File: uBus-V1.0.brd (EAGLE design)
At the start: 160 x 100 mm, 20 parts, among them J1 FTDI, U1 MIC5219 3.3V, U2 FTS31XS-U

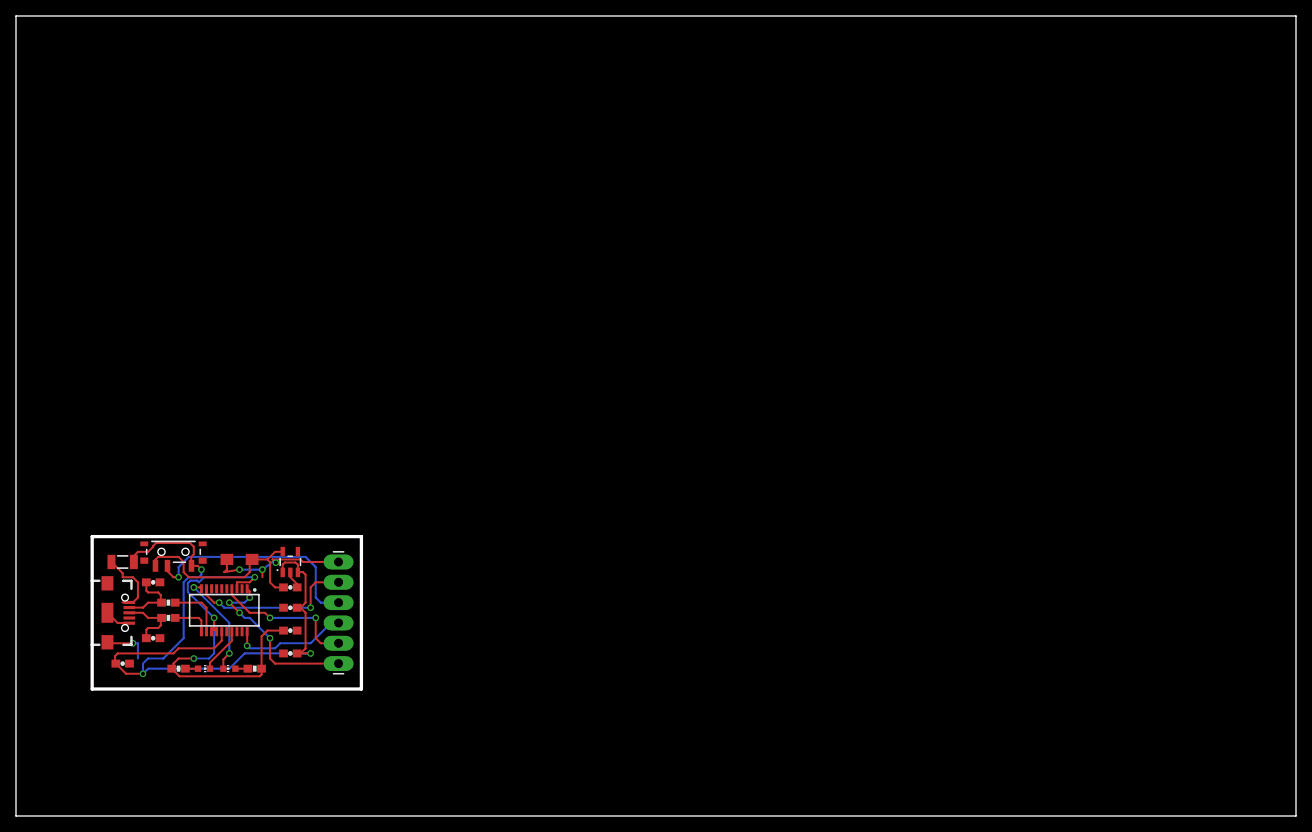
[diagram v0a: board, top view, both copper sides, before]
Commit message: Placa mandada a fabrica
Logos añadidos
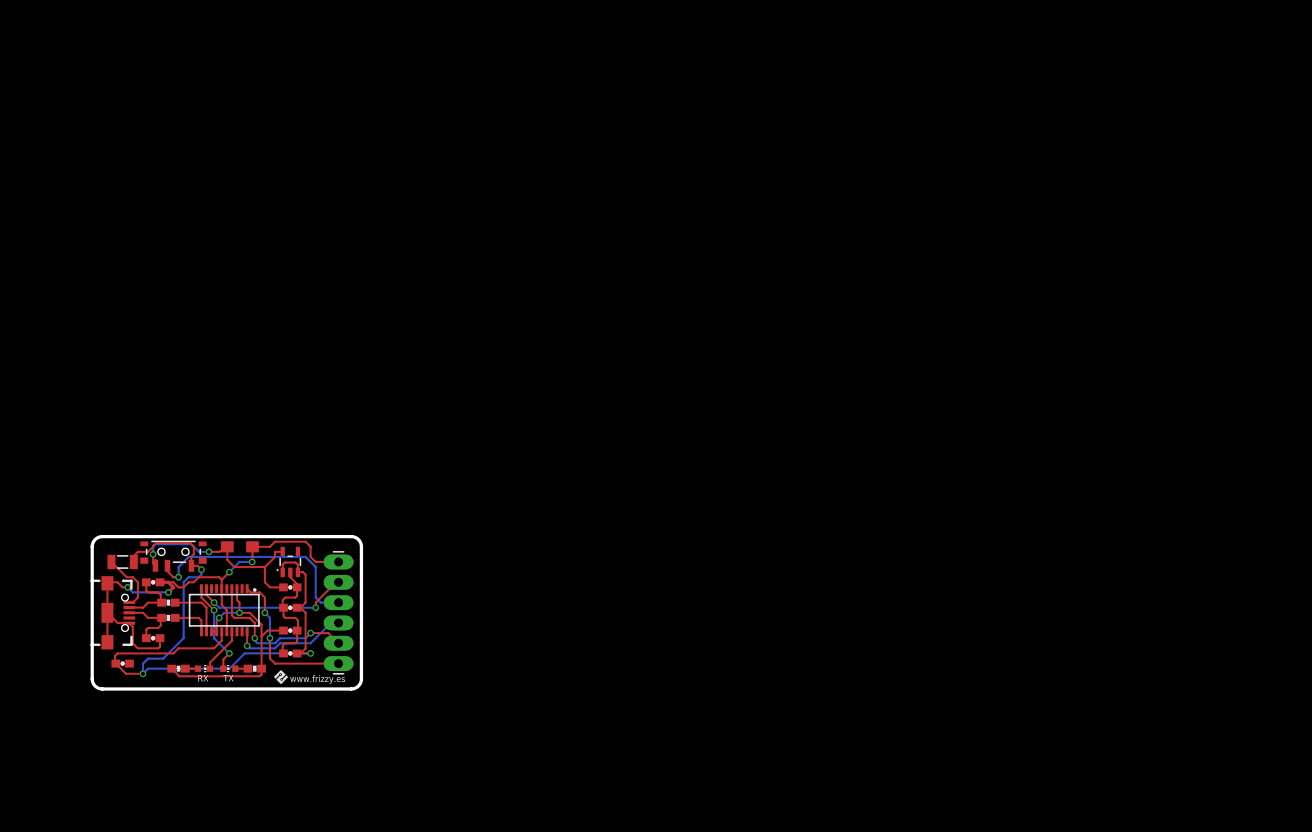
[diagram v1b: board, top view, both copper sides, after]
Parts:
- added U$1: (no value), SparkFun-Aesthetics:OSHW-LOGO-S
- moved C9 1.58 mm to (28.0, 33.6), turned to 0 degrees
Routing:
- net GND: track 29.5 -> 79.5 mm
- net VCCIO: track 50.9 -> 32.8 mm, vias 3 -> 2
- net DTR: track 22.3 -> 19.4 mm, vias 4 -> 2
- net RXD: track 18.1 -> 20.5 mm
- net 3.3V: track 25.6 -> 27.9 mm, vias 0 -> 2
- net CBUS2: track 13.3 -> 11.7 mm
- net N$11: track 8.74 -> 7.60 mm
- net CTS: track 20.7 -> 19.6 mm
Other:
- board size 160 x 100 mm -> 33.7 x 19 mm
- board text added: "RX"
- board text added: "TX"
- board text added: "www.frizzy.es"
